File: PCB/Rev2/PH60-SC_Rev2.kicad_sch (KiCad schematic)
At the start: 43 parts, among them J1 USB_C_Receptacle_USB2.0_14P, J2 Conn_01x02_Pin, J3 Conn_01x02_Pin, U1 nRF52840, X1 32.768kHz, X2 Crystal_Generic

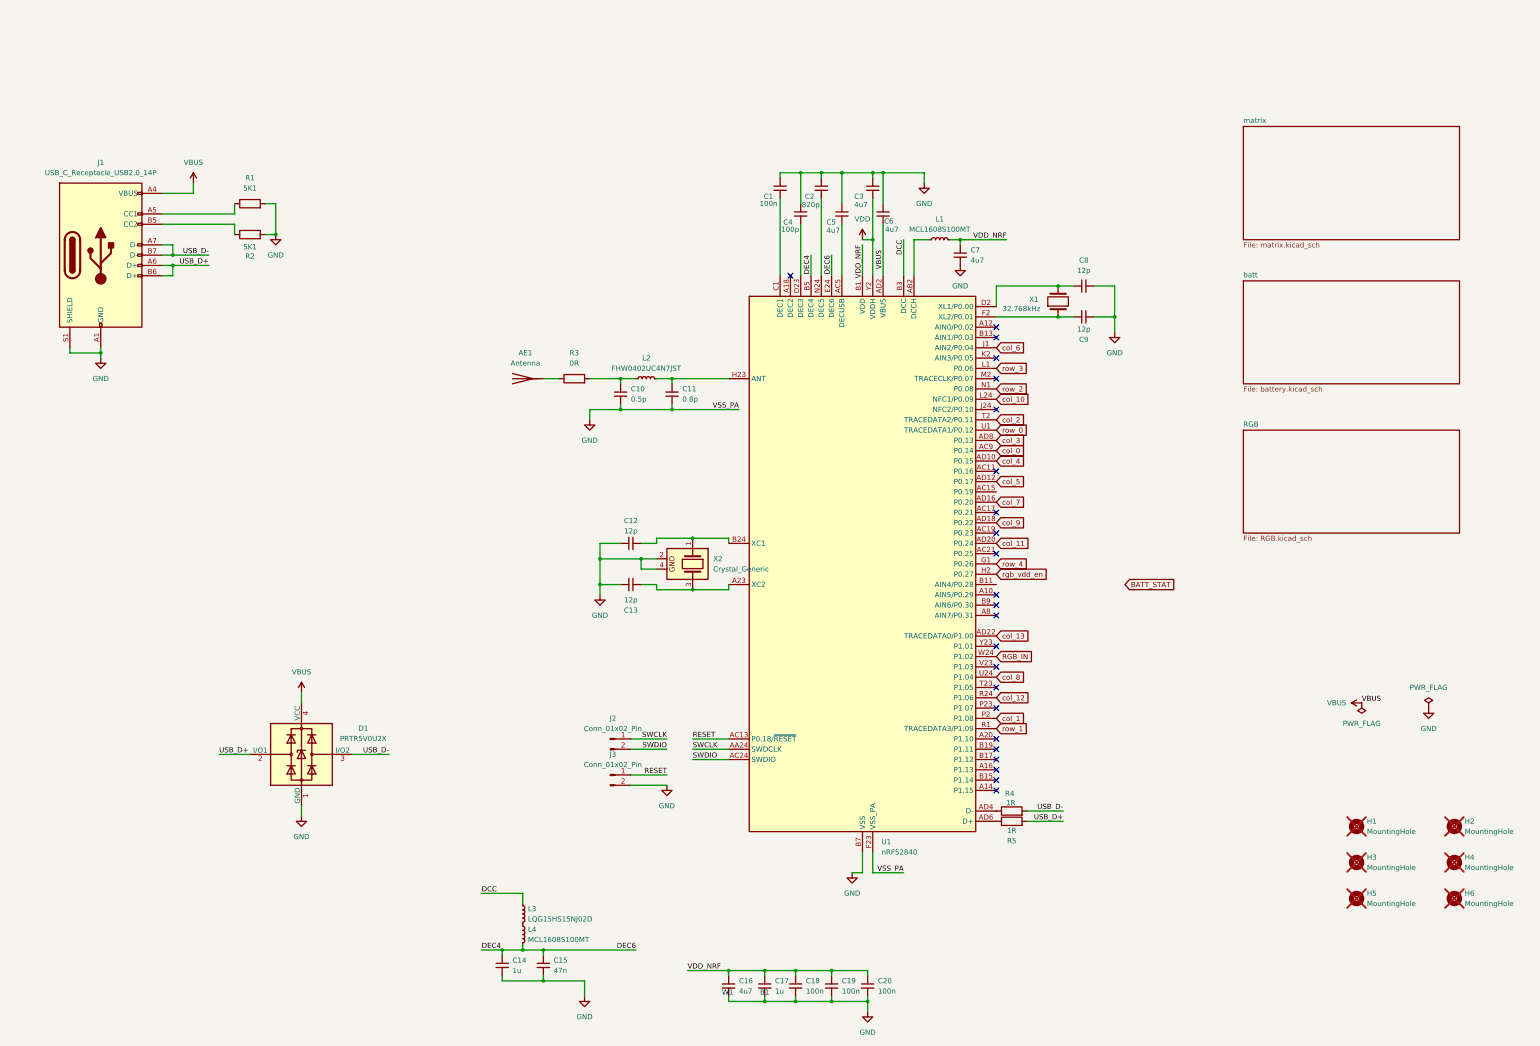
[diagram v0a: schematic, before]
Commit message: sc2最终审核（nayat）
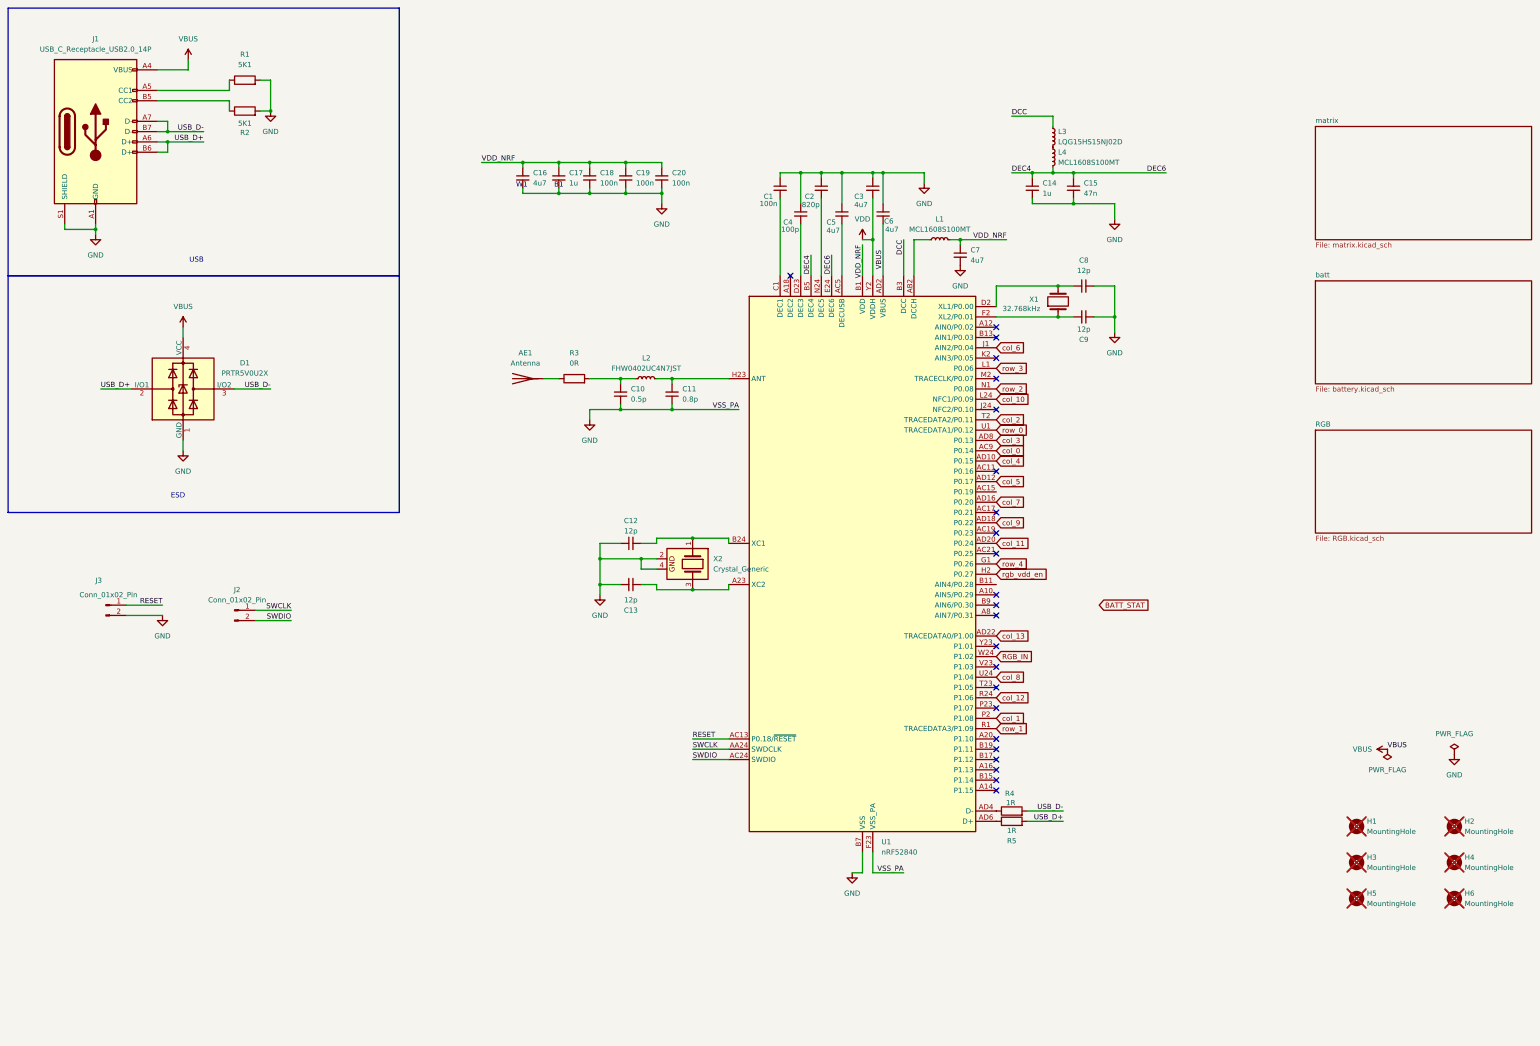
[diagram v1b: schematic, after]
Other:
- note added: "ESD"
- note added: "USB"
- moved on the sheet: C14, C15, C16, C17, C18, C19, C20, D1, J1, J2, J3, L3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
